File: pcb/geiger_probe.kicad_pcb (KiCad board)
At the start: 4 copper layers, 146.1 x 29.9 mm, 115 parts, among them IC1 LT8606IDC#TRPBF, IC2 ATA6561-GAQW-N, IC8 MCP79410T-I_MS, J1 Conn_01x05_Socket, J2 TC2030, Q1 DMN3404L, Q2 BSS138, U1 STM32L432KCUx, U2 MCP1700x-330xxMB, U3 INA186A4IDCKR, U701 GAQY212GS, U702 GAQY212GS, Y1 32,768kHz

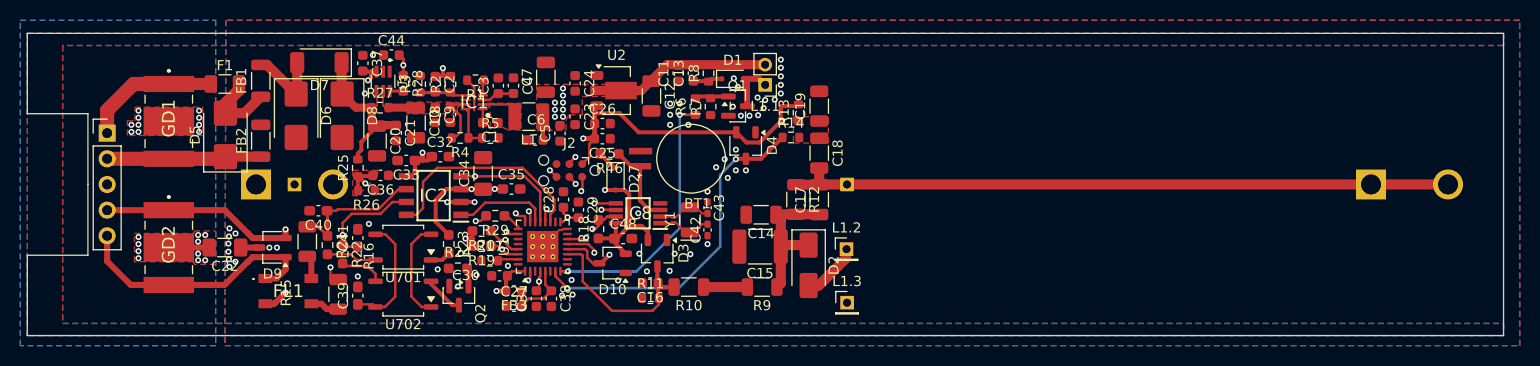
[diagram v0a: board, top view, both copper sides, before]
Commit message: Finished routing, needs polishing
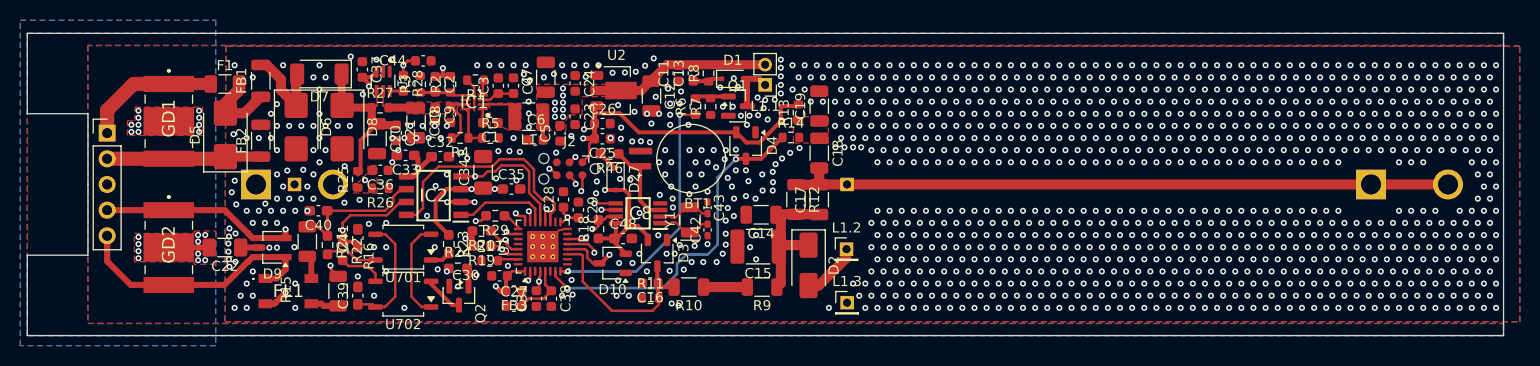
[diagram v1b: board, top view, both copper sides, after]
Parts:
- moved C44 3.20 mm to (155.5, 64.9), turned to 180 degrees
- moved R26 1.39 mm to (151.2, 77.5)
- moved R25 1.15 mm to (149.0, 76.6)
- moved D6 1.12 mm to (142.9, 71.4)
- moved D7 1.12 mm to (145.2, 66.2)
- moved D8 1.12 mm to (147.4, 71.4)
- moved C37 0.63 mm to (149.4, 65.7)
- moved C33 0.51 mm to (153.7, 74.2)
- moved C36 0.50 mm to (151.2, 75.7)
- moved R22 0.33 mm to (147.5, 83.7)
- moved R15 0.32 mm to (147.1, 87.7)
- moved C20 0.22 mm to (150.9, 72.6)
- moved C15 0.20 mm to (188.6, 83.2)
- moved J2 0.17 mm to (169.9, 75.5)
- moved C34 0.11 mm to (161.4, 75.9)
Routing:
- net /MCU/VIN_SENSE: track 48.4 -> 43.8 mm
- net /CAN_BUS/CAN_STBY: track 21.8 -> 23.6 mm
- net /MCU/EN_I_SENS: track 54.1 -> 52.6 mm
- net +3.3V: track 106.9 -> 105.5 mm
- net /CAN_BUS/CAN_RX: track 18.1 -> 19.6 mm
- net /PROTECTION/V_zas: track 16.7 -> 17.9 mm
- net Net-(D6-K): track 7.83 -> 8.93 mm
- net /MCU/I_SENS: track 52.6 -> 51.5 mm
- net GND: vias 57 -> 1223
